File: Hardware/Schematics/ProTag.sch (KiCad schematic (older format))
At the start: 57 parts, among them IC1 MC3216, IC2 QN9090THN_001Z, J1 Conn_01x01_Female, J10 TEST_POINT, J11 TEST_POINT, J12 TEST_POINT, J13 TEST_POINT, J14 TEST_POINT, J15 TEST_POINT, J16 TEST_POINT, J17 TEST_POINT, J18 TEST_POINT, J19 TEST_POINT, J2 TEST_POINT, J3 TEST_POINT, J4 TEST_POINT, J5 TEST_POINT, J6 TEST_POINT, J7 TEST_POINT, J8 TEST_POINT, J9 TEST_POINT, Q1 BC818W, SW1 SW_SPST, U1 TC2185-3.3VxCTTR, Y1 NX2012SA-32.768K-STD-MUB-1, Y2 NX2016SA-32M-EXS00A-CS06465

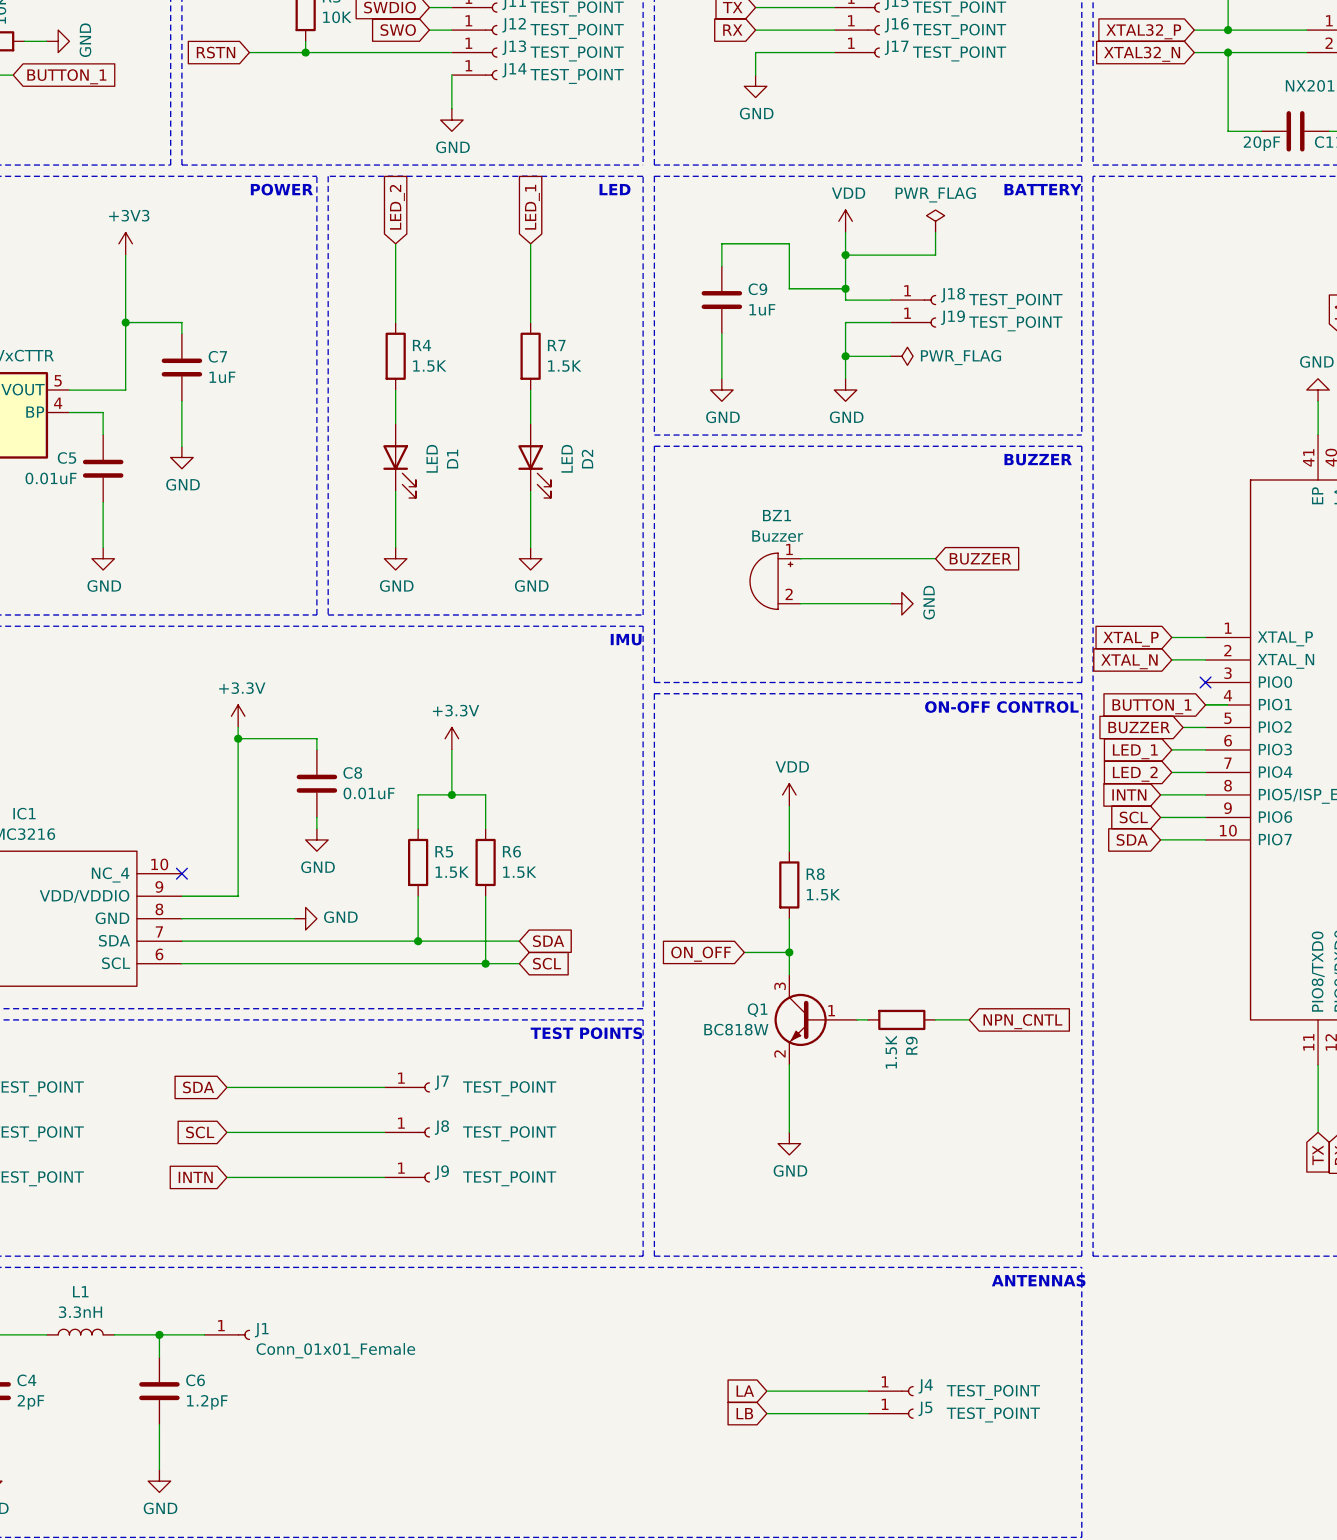
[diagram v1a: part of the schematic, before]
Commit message: Add files via upload
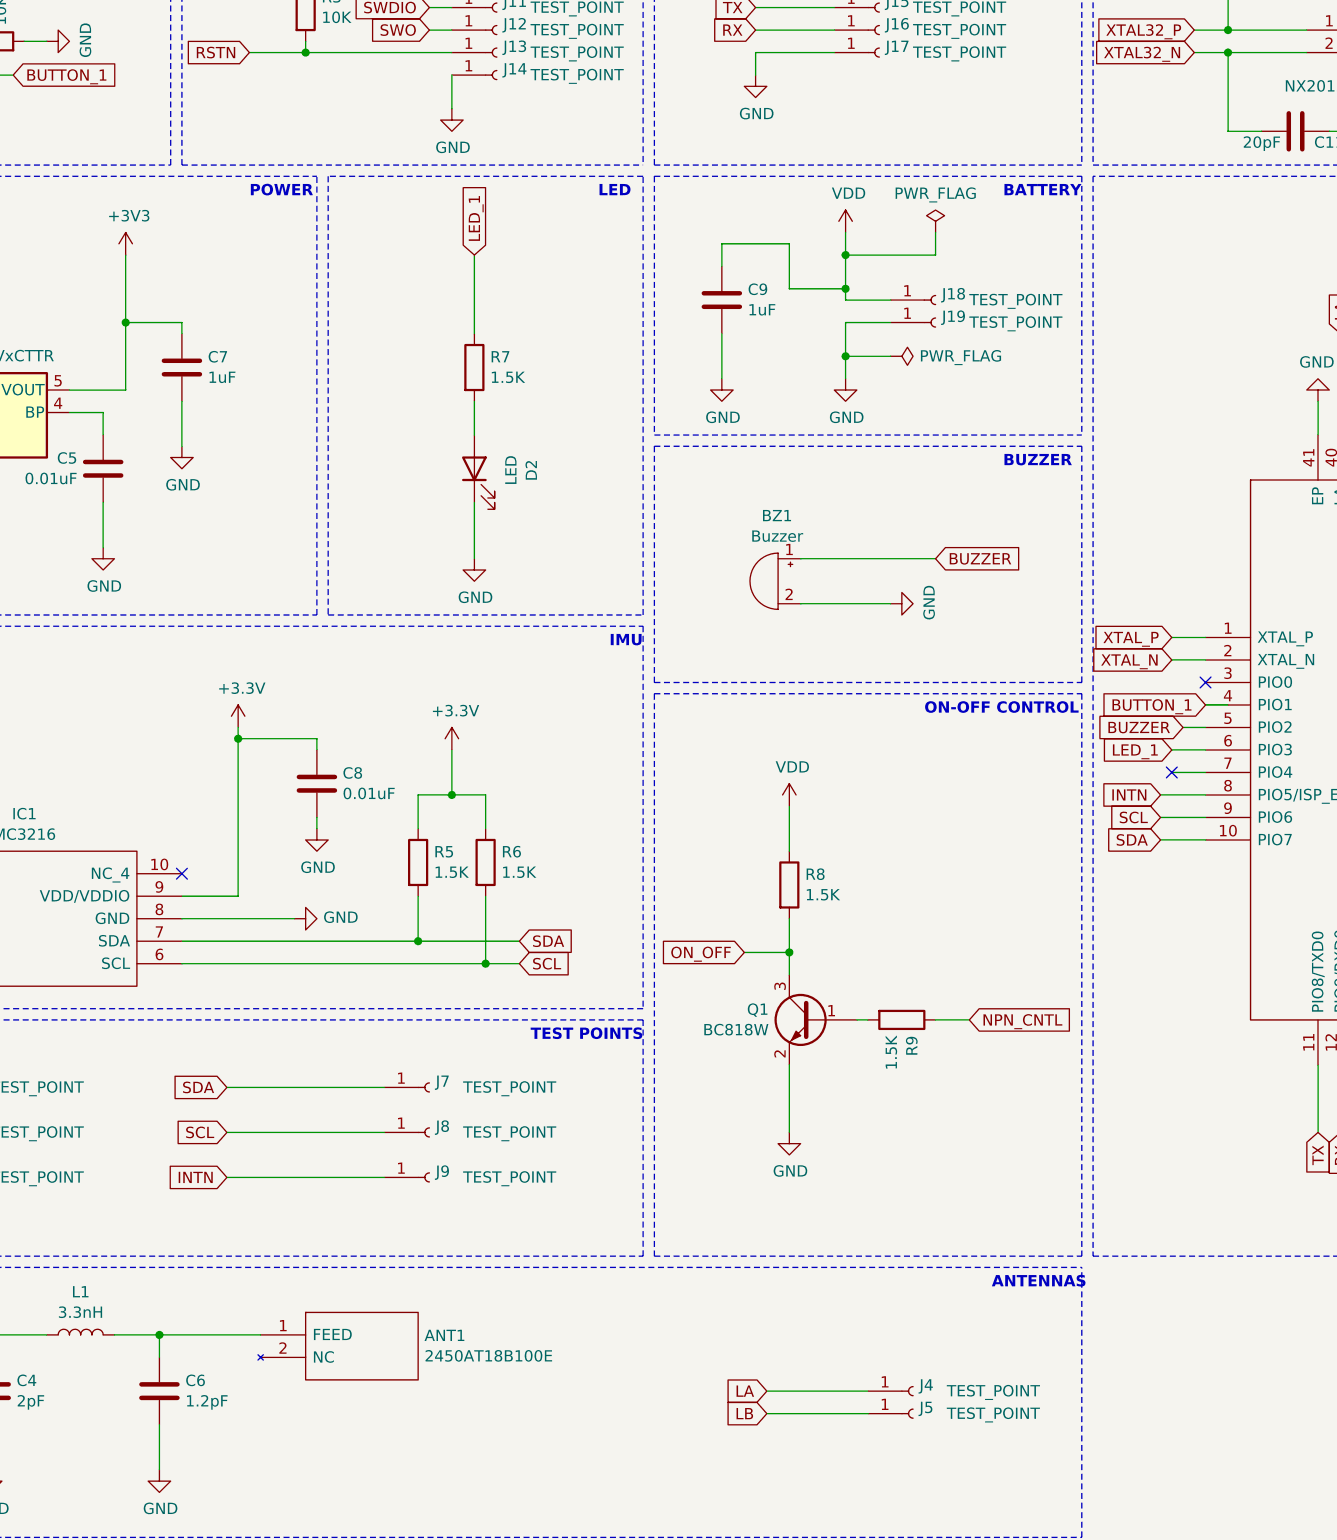
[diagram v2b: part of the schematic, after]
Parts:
- removed D1: LED, Diode_SMD:D_0201_0603Metric, symbol Device:LED
- removed J1: Conn_01x01_Female, TestPoint:TestPoint_Pad_D1.0mm, symbol Connector:Conn_01x01_Female
- removed R4: 1.5K, Resistor_SMD:R_0201_0603Metric, symbol Device:R
- added ANT1: 2450AT18B100E, ASSETS:ANTC3216X140N, symbol Regular_Use:2450AT18B100E
- J10, J11, J12, J13, J14, J15, J16, J17, J18, J19, J2, J3, J4, J5, J6, J7, J8, J9: footprint TestPoint:TestPoint_Pad_D1.0mm -> ASSETS:testpoint_0.3mm
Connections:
- net at C6.1, L1.2: now also ANT1.1 (FEED)
- net LED_2: no longer names the net of IC2.7 (PIO4)
- no-connect marks 13 -> 14
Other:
- moved on the sheet: D2, R7
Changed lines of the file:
@@
 Text Notes 8650 600  0    50   ~ 10
 XTAL 32KHz
-Text GLabel 7350 4350 0    50   Input ~ 0
-LED_2
 Wire Wire Line
 	7350 4350 7500 4350
@@
 L Device:R R7
 U 1 1 609D2878
-P 4500 2500
-F 0 "R7" H 4570 2546 50  0000 L CNN
-F 1 "1.5K" H 4570 2455 50  0000 L CNN
-F 2 "Resistor_SMD:R_0201_0603Metric" V 4430 2500 50  0001 C CNN
-F 3 "~" H 4500 2500 50  0001 C CNN
-	1    4500 2500
+P 4250 2550
+F 0 "R7" H 4320 2596 50  0000 L CNN
+F 1 "1.5K" H 4320 2505 50  0000 L CNN
+F 2 "Resistor_SMD:R_0201_0603Metric" V 4180 2550 50  0001 C CNN
+F 3 "~" H 4250 2550 50  0001 C CNN
+	1    4250 2550
 	1    0    0    -1
 $EndComp
@@
 L Device:LED D2
 U 1 1 609D37A3
-P 4500 2950
-F 0 "D2" H 4493 2695 50  0000 C CNN
-F 1 "LED" H 4493 2786 50  0000 C CNN
-F 2 "Diode_SMD:D_0201_0603Metric" H 4500 2950 50  0001 C CNN
-F 3 "~" H 4500 2950 50  0001 C CNN
-	1    4500 2950
+P 4250 3000
+F 0 "D2" H 4243 2745 50  0000 C CNN
+F 1 "LED" H 4243 2836 50  0000 C CNN
+F 2 "Diode_SMD:D_0201_0603Metric" H 4250 3000 50  0001 C CNN
+F 3 "~" H 4250 3000 50  0001 C CNN
+	1    4250 3000
 	0    -1   -1   0
 $EndComp
 Wire Wire Line
-	4500 2800 4500 2650
+	4250 2850 4250 2700
 $Comp
 L power:GND #PWR021
 U 1 1 609D93AC
-P 4500 3350
-F 0 "#PWR021" H 4500 3100 50  0001 C CNN
-F 1 "GND" H 4505 3177 50  0000 C CNN
-F 2 "" H 4500 3350 50  0001 C CNN
-F 3 "" H 4500 3350 50  0001 C CNN
-	1    4500 3350
-	1    0    0    -1
-$EndComp
-Wire Wire Line
-	4500 2350 4500 2000
+P 4250 3400
+F 0 "#PWR021" H 4250 3150 50  0001 C CNN
+F 1 "GND" H 4255 3227 50  0000 C CNN
+F 2 "" H 4250 3400 50  0001 C CNN
+F 3 "" H 4250 3400 50  0001 C CNN
+	1    4250 3400
+	1    0    0    -1
+$EndComp
+Wire Wire Line
+	4250 2400 4250 2050
 Wire Notes Line
 	6950 7750 6950 6550
@@
 Wire Wire Line
 	1550 6850 1150 6850
-$Comp
-L Connector:Conn_01x01_Female J1
-U 1 1 609FC71F
-P 3250 6850
-F 0 "J1" H 3278 6876 50  0000 L CNN
-F 1 "Conn_01x01_Female" H 3278 6785 50  0000 L CNN
-F 2 "TestPoint:TestPoint_Pad_D1.0mm" H 3250 6850 50  0001 C CNN
-F 3 "~" H 3250 6850 50  0001 C CNN
-	1    3250 6850
-	1    0    0    -1
-$EndComp
 Connection ~ 2850 6850
-Wire Wire Line
-	2850 6850 3050 6850
 Wire Wire Line
 	2850 6850 2650 6850
@@
 	5000 3650 5000 1700
 Wire Wire Line
-	4500 3100 4500 3350
-$Comp
-L Device:R R4
-U 1 1 60A4C794
-P 3900 2500
-F 0 "R4" H 3970 2546 50  0000 L CNN
-F 1 "1.5K" H 3970 2455 50  0000 L CNN
-F 2 "Resistor_SMD:R_0201_0603Metric" V 3830 2500 50  0001 C CNN
-F 3 "~" H 3900 2500 50  0001 C CNN
-	1    3900 2500
-	1    0    0    -1
-$EndComp
-$Comp
-L Device:LED D1
-U 1 1 60A4C79A
-P 3900 2950
-F 0 "D1" H 3893 2695 50  0000 C CNN
-F 1 "LED" H 3893 2786 50  0000 C CNN
-F 2 "Diode_SMD:D_0201_0603Metric" H 3900 2950 50  0001 C CNN
-F 3 "~" H 3900 2950 50  0001 C CNN
-	1    3900 2950
-	0    -1   -1   0
-$EndComp
-Wire Wire Line
-	3900 2800 3900 2650
-$Comp
-L power:GND #PWR018
-U 1 1 60A4C7A1
-P 3900 3350
-F 0 "#PWR018" H 3900 3100 50  0001 C CNN
-F 1 "GND" H 3905 3177 50  0000 C CNN
-F 2 "" H 3900 3350 50  0001 C CNN
-F 3 "" H 3900 3350 50  0001 C CNN
-	1    3900 3350
-	1    0    0    -1
-$EndComp
-Wire Wire Line
-	3900 2350 3900 2000
-Wire Wire Line
-	3900 3100 3900 3350
-Text GLabel 4500 2000 1    50   Input ~ 0
+	4250 3150 4250 3400
+Text GLabel 4250 2050 1    50   Input ~ 0
 LED_1
-Text GLabel 3900 2000 1    50   Input ~ 0
-LED_2
 Text Notes 4800 1800 0    50   ~ 10
 LED
@@
 F 0 "J10" H 4378 876 50  0000 L CNN
 F 1 "TEST_POINT" H 4500 850 50  0000 L CNN
-F 2 "TestPoint:TestPoint_Pad_D1.0mm" H 4350 850 50  0001 C CNN
+F 2 "ASSETS:testpoint_0.3mm" H 4350 850 50  0001 C CNN
 F 3 "~" H 4350 850 50  0001 C CNN
 	1    4350 850
@@
 F 0 "J11" H 4378 976 50  0000 L CNN
 F 1 "TEST_POINT" H 4500 950 50  0000 L CNN
-F 2 "TestPoint:TestPoint_Pad_D1.0mm" H 4350 950 50  0001 C CNN
+F 2 "ASSETS:testpoint_0.3mm" H 4350 950 50  0001 C CNN
 F 3 "~" H 4350 950 50  0001 C CNN
 	1    4350 950
@@
 F 0 "J12" H 4378 1076 50  0000 L CNN
 F 1 "TEST_POINT" H 4500 1050 50  0000 L CNN
-F 2 "TestPoint:TestPoint_Pad_D1.0mm" H 4350 1050 50  0001 C CNN
+F 2 "ASSETS:testpoint_0.3mm" H 4350 1050 50  0001 C CNN
 F 3 "~" H 4350 1050 50  0001 C CNN
 	1    4350 1050
@@
 F 0 "J13" H 4378 1176 50  0000 L CNN
 F 1 "TEST_POINT" H 4500 1150 50  0000 L CNN
-F 2 "TestPoint:TestPoint_Pad_D1.0mm" H 4350 1150 50  0001 C CNN
+F 2 "ASSETS:testpoint_0.3mm" H 4350 1150 50  0001 C CNN
 F 3 "~" H 4350 1150 50  0001 C CNN
 	1    4350 1150
@@
 F 0 "J14" H 4378 1276 50  0000 L CNN
 F 1 "TEST_POINT" H 4500 1250 50  0000 L CNN
-F 2 "TestPoint:TestPoint_Pad_D1.0mm" H 4350 1250 50  0001 C CNN
+F 2 "ASSETS:testpoint_0.3mm" H 4350 1250 50  0001 C CNN
 F 3 "~" H 4350 1250 50  0001 C CNN
 	1    4350 1250
@@
 F 0 "J15" H 6078 976 50  0000 L CNN
 F 1 "TEST_POINT" H 6200 950 50  0000 L CNN
-F 2 "TestPoint:TestPoint_Pad_D1.0mm" H 6050 950 50  0001 C CNN
+F 2 "ASSETS:testpoint_0.3mm" H 6050 950 50  0001 C CNN
 F 3 "~" H 6050 950 50  0001 C CNN
 	1    6050 950
@@
 F 0 "J16" H 6078 1076 50  0000 L CNN
 F 1 "TEST_POINT" H 6200 1050 50  0000 L CNN
-F 2 "TestPoint:TestPoint_Pad_D1.0mm" H 6050 1050 50  0001 C CNN
+F 2 "ASSETS:testpoint_0.3mm" H 6050 1050 50  0001 C CNN
 F 3 "~" H 6050 1050 50  0001 C CNN
 	1    6050 1050
@@
 F 0 "J17" H 6078 1176 50  0000 L CNN
 F 1 "TEST_POINT" H 6200 1150 50  0000 L CNN
-F 2 "TestPoint:TestPoint_Pad_D1.0mm" H 6050 1150 50  0001 C CNN
+F 2 "ASSETS:testpoint_0.3mm" H 6050 1150 50  0001 C CNN
 F 3 "~" H 6050 1150 50  0001 C CNN
 	1    6050 1150
@@
 F 0 "J8" H 4078 5976 50  0000 L CNN
 F 1 "TEST_POINT" H 4200 5950 50  0000 L CNN
-F 2 "TestPoint:TestPoint_Pad_D1.0mm" H 4050 5950 50  0001 C CNN
+F 2 "ASSETS:testpoint_0.3mm" H 4050 5950 50  0001 C CNN
 F 3 "~" H 4050 5950 50  0001 C CNN
 	1    4050 5950
@@
 F 0 "J9" H 4078 6176 50  0000 L CNN
 F 1 "TEST_POINT" H 4200 6150 50  0000 L CNN
-F 2 "TestPoint:TestPoint_Pad_D1.0mm" H 4050 6150 50  0001 C CNN
+F 2 "ASSETS:testpoint_0.3mm" H 4050 6150 50  0001 C CNN
 F 3 "~" H 4050 6150 50  0001 C CNN
 	1    4050 6150
@@
 F 0 "J2" H 1978 5776 50  0000 L CNN
 F 1 "TEST_POINT" H 2100 5750 50  0000 L CNN
-F 2 "TestPoint:TestPoint_Pad_D1.0mm" H 1950 5750 50  0001 C CNN
+F 2 "ASSETS:testpoint_0.3mm" H 1950 5750 50  0001 C CNN
 F 3 "~" H 1950 5750 50  0001 C CNN
 	1    1950 5750
@@
 F 0 "J7" H 4078 5776 50  0000 L CNN
 F 1 "TEST_POINT" H 4200 5750 50  0000 L CNN
-F 2 "TestPoint:TestPoint_Pad_D1.0mm" H 4050 5750 50  0001 C CNN
+F 2 "ASSETS:testpoint_0.3mm" H 4050 5750 50  0001 C CNN
 F 3 "~" H 4050 5750 50  0001 C CNN
 	1    4050 5750
@@
 F 0 "J3" H 1978 5976 50  0000 L CNN
 F 1 "TEST_POINT" H 2100 5950 50  0000 L CNN
-F 2 "TestPoint:TestPoint_Pad_D1.0mm" H 1950 5950 50  0001 C CNN
+F 2 "ASSETS:testpoint_0.3mm" H 1950 5950 50  0001 C CNN
 F 3 "~" H 1950 5950 50  0001 C CNN
 	1    1950 5950
@@
 F 0 "J6" H 1978 6176 50  0000 L CNN
 F 1 "TEST_POINT" H 2100 6150 50  0000 L CNN
-F 2 "TestPoint:TestPoint_Pad_D1.0mm" H 1950 6150 50  0001 C CNN
+F 2 "ASSETS:testpoint_0.3mm" H 1950 6150 50  0001 C CNN
 F 3 "~" H 1950 6150 50  0001 C CNN
 	1    1950 6150
@@
 F 0 "J18" H 6328 2276 50  0000 L CNN
 F 1 "TEST_POINT" H 6450 2250 50  0000 L CNN
-F 2 "TestPoint:TestPoint_Pad_D1.0mm" H 6300 2250 50  0001 C CNN
+F 2 "ASSETS:testpoint_0.3mm" H 6300 2250 50  0001 C CNN
 F 3 "~" H 6300 2250 50  0001 C CNN
 	1    6300 2250
@@
 F 0 "J19" H 6328 2376 50  0000 L CNN
 F 1 "TEST_POINT" H 6450 2350 50  0000 L CNN
-F 2 "TestPoint:TestPoint_Pad_D1.0mm" H 6300 2350 50  0001 C CNN
+F 2 "ASSETS:testpoint_0.3mm" H 6300 2350 50  0001 C CNN
 F 3 "~" H 6300 2350 50  0001 C CNN
 	1    6300 2350
@@
 F 0 "J4" H 6228 7126 50  0000 L CNN
 F 1 "TEST_POINT" H 6350 7100 50  0000 L CNN
-F 2 "TestPoint:TestPoint_Pad_D1.0mm" H 6200 7100 50  0001 C CNN
+F 2 "ASSETS:testpoint_0.3mm" H 6200 7100 50  0001 C CNN
 F 3 "~" H 6200 7100 50  0001 C CNN
 	1    6200 7100
@@
 F 0 "J5" H 6228 7226 50  0000 L CNN
 F 1 "TEST_POINT" H 6350 7200 50  0000 L CNN
-F 2 "TestPoint:TestPoint_Pad_D1.0mm" H 6200 7200 50  0001 C CNN
+F 2 "ASSETS:testpoint_0.3mm" H 6200 7200 50  0001 C CNN
 F 3 "~" H 6200 7200 50  0001 C CNN
 	1    6200 7200
 	1    0    0    -1
 $EndComp
+$Comp
+L Regular_Use:2450AT18B100E ANT1
+U 1 1 60ACE974
+P 3300 6850
+F 0 "ANT1" H 4028 6846 50  0000 L CNN
+F 1 "2450AT18B100E" H 4028 6755 50  0000 L CNN
+F 2 "ASSETS:ANTC3216X140N" H 4050 6950 50  0001 L CNN
+F 3 "https://www.johansontechnology.com/datasheets/2450AT18B100/2450AT18B100.pdf" H 4050 6850 50  0001 L CNN
+F 4 "Antennas 2.45GHz ANTENNA" H 4050 6750 50  0001 L CNN "Description"
+F 5 "1.4" H 4050 6650 50  0001 L CNN "Height"
+F 6 "609-2450AT18B100E" H 4050 6550 50  0001 L CNN "Mouser Part Number"
+F 7 "https://www.mouser.co.uk/ProductDetail/Johanson-Technology/2450AT18B100E/?qs=yCnrNFeXz%252Bh5MFsFIXGZGA%3D%3D" H 4050 6450 50  0001 L CNN "Mouser Price/Stock"
+F 8 "JOHANSON TECHNOLOGY" H 4050 6350 50  0001 L CNN "Manufacturer_Name"
+F 9 "2450AT18B100E" H 4050 6250 50  0001 L CNN "Manufacturer_Part_Number"
+	1    3300 6850
+	1    0    0    -1
+$EndComp
+Wire Wire Line
+	2850 6850 3300 6850
+NoConn ~ 7350 4350
 $EndSCHEMATC
